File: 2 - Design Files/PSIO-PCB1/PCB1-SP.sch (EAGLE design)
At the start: 40 parts

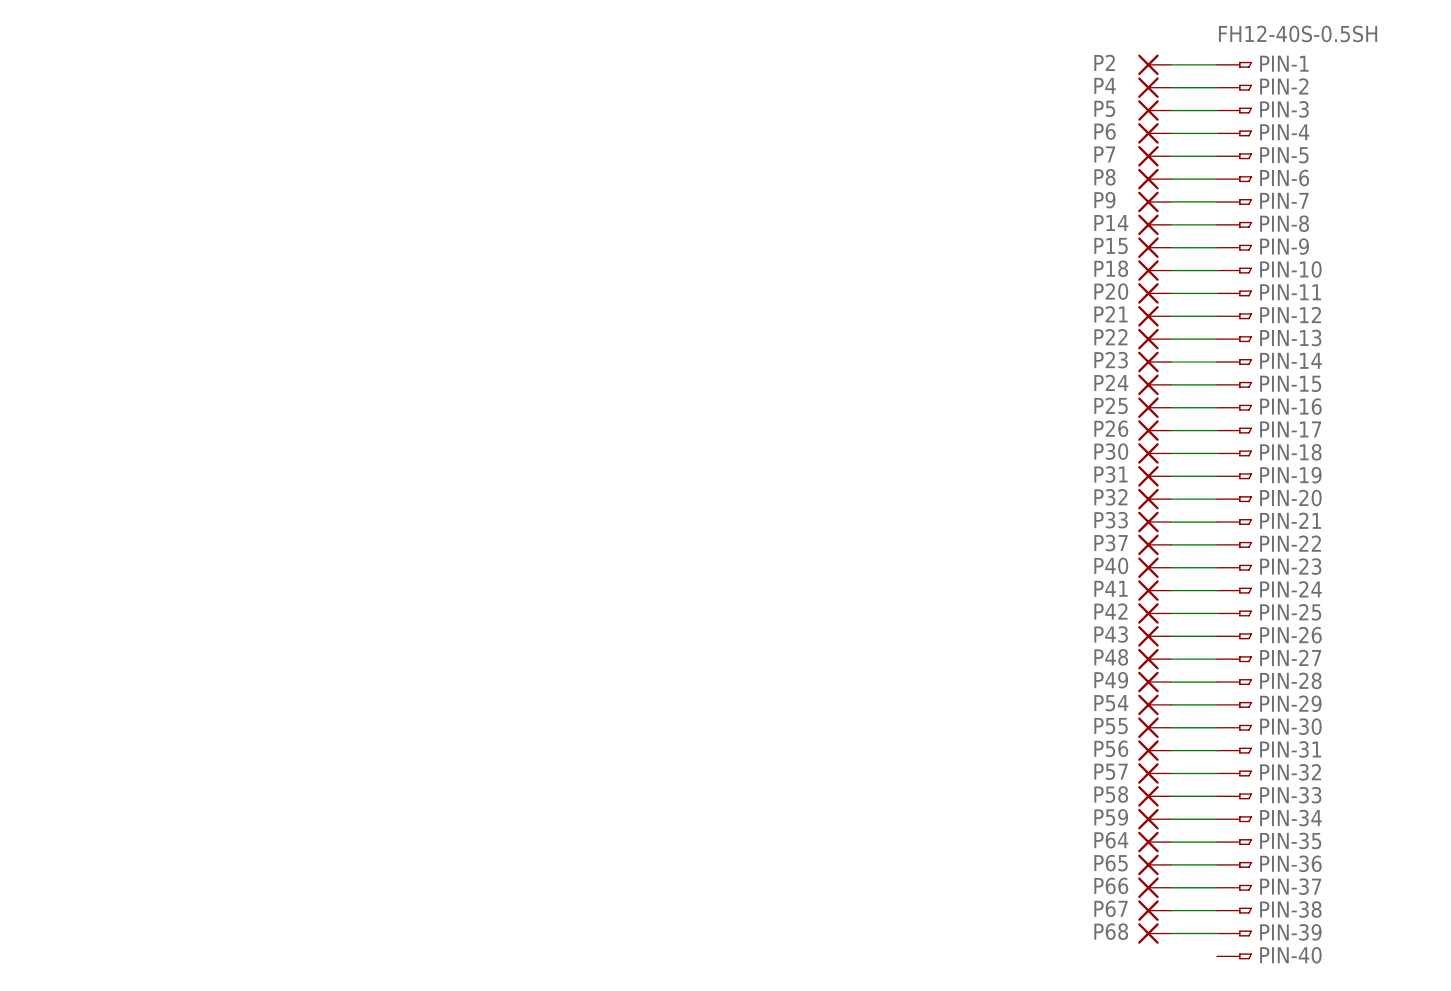
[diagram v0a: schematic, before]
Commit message: finished first PCB
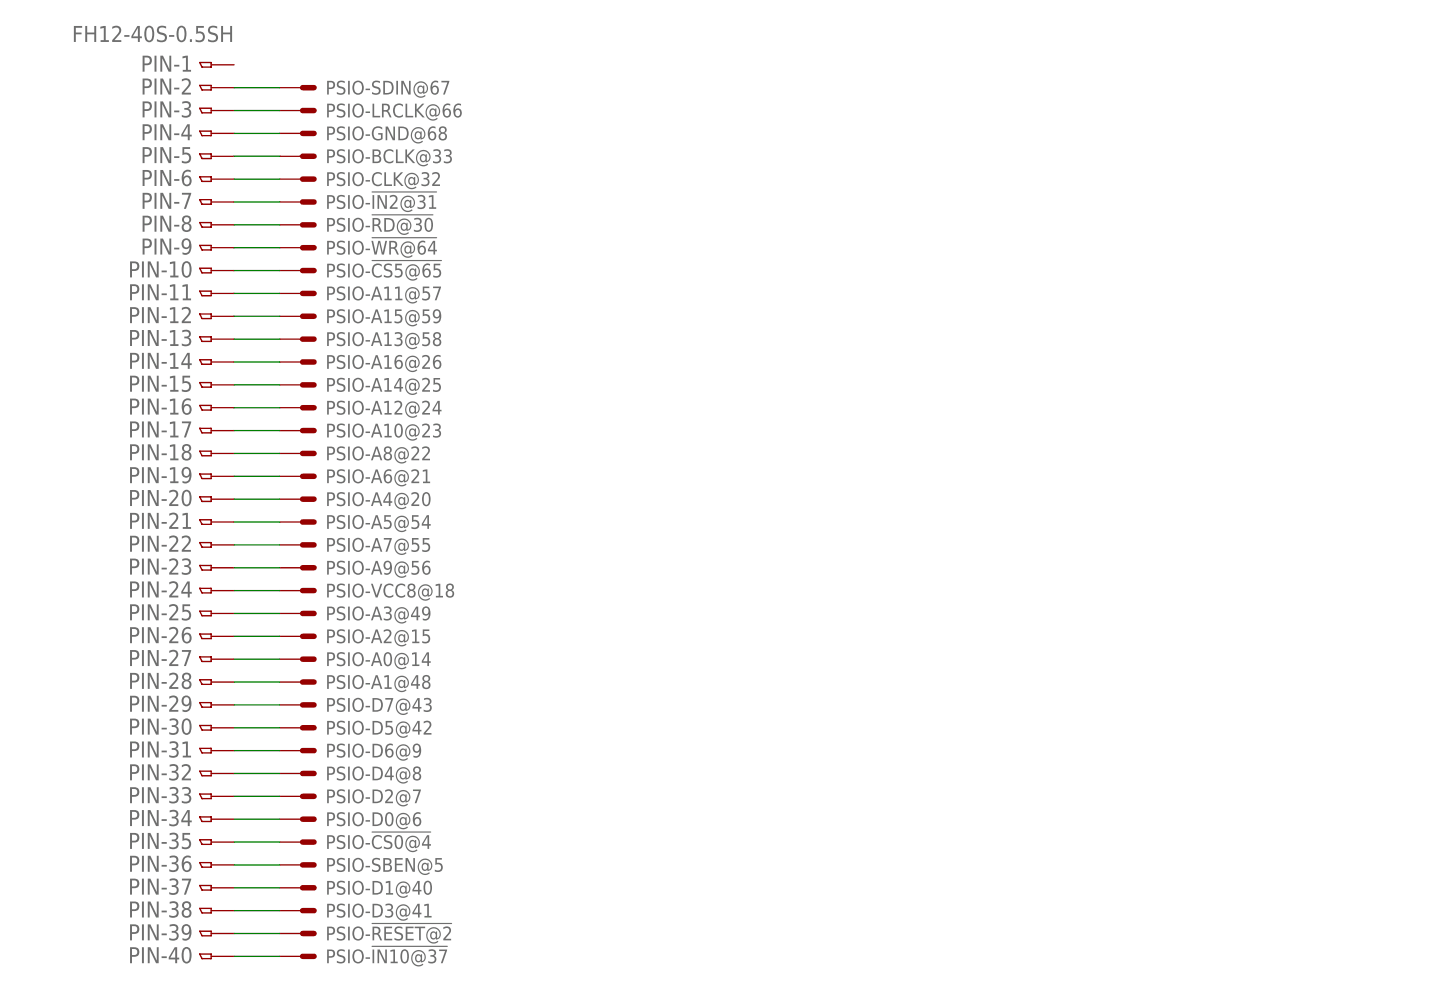
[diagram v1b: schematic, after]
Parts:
- removed P14, P15, P18, P2, P20, P21, P22, P23, P24, P25, P26, P30, P31, P32, P33, P37, P4, P40, P41, P42, P43, P48, P49, P5, P54, P55, P56, P57, P58, P59, P6, P64, P65, P66, P67, P68, P7, P8, P9: (no value), wirepad:1,6/0,8
- added PSIO: PIOCONNPIOCONN-S, pixel:PIOCONNPIOCONN-S
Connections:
- net N$1: now also PIN-40.1, PSIO-!IN10@37.S; no longer P2.P, PIN-1.1
- net N$10: now also PIN-31.1, PSIO-D6@9.S; no longer P14.P, PIN-8.1
- net N$11: now also PIN-30.1, PSIO-D5@42.S; no longer P15.P, PIN-9.1
- net N$12: now also PIN-29.1, PSIO-D7@43.S; no longer P18.P, PIN-10.1
- net N$13: now also PIN-28.1, PSIO-A1@48.S; no longer P20.P, PIN-11.1
- net N$14: now also PIN-27.1, PSIO-A0@14.S; no longer P21.P, PIN-12.1
- net N$15: now also PIN-26.1, PSIO-A2@15.S; no longer P23.P, PIN-14.1
- net N$16: now also PIN-25.1, PSIO-A3@49.S; no longer P24.P, PIN-15.1
- net N$17: now also PIN-24.1, PSIO-VCC8@18.S; no longer P25.P, PIN-16.1
- net N$18: now also PIN-2.1, PSIO-SDIN@67.S; no longer P26.P, PIN-17.1
- net N$19: now also PIN-3.1, PSIO-LRCLK@66.S; no longer P30.P, PIN-18.1
- net N$2: now also PIN-39.1, PSIO-!RESET@2.S; no longer P6.P, PIN-4.1
- net N$20: now also PIN-4.1, PSIO-GND@68.S; no longer P31.P, PIN-19.1
- net N$21: now also PIN-5.1, PSIO-BCLK@33.S; no longer P32.P, PIN-20.1
- net N$22: now also PIN-6.1, PSIO-CLK@32.S; no longer P33.P, PIN-21.1
- net N$23: now also PIN-7.1, PSIO-!IN2@31.S; no longer P37.P, PIN-22.1
- net N$24: now also PIN-8.1, PSIO-!RD@30.S; no longer P40.P, PIN-23.1
- net N$25: now also PIN-9.1, PSIO-!WR@64.S; no longer P41.P, PIN-24.1
- net N$26: now also PIN-10.1, PSIO-!CS5@65.S; no longer P48.P, PIN-27.1
- net N$27: now also PIN-23.1, PSIO-A9@56.S; no longer P49.P, PIN-28.1
- net N$28: now also PIN-11.1, PSIO-A11@57.S; no longer P54.P, PIN-29.1
- net N$29: now also PIN-22.1, PSIO-A7@55.S; no longer P55.P, PIN-30.1
- net N$3: now also PIN-38.1, PSIO-D3@41.S; no longer P42.P, PIN-25.1
- net N$30: now also PIN-21.1, PSIO-A5@54.S; no longer P56.P, PIN-31.1
- net N$31: now also PIN-12.1, PSIO-A15@59.S; no longer P57.P, PIN-32.1
- net N$32: now also PIN-13.1, PSIO-A13@58.S; no longer P58.P, PIN-33.1
- net N$33: now also PIN-20.1, PSIO-A4@20.S; no longer P59.P, PIN-34.1
- net N$34: now also PIN-14.1, PSIO-A16@26.S; no longer P64.P, PIN-35.1
- net N$35: now also PIN-19.1, PSIO-A6@21.S; no longer P65.P, PIN-36.1
- net N$36: now also PIN-15.1, PSIO-A14@25.S; no longer P66.P, PIN-37.1
- net N$37: now also PIN-16.1, PSIO-A12@24.S; no longer P67.P, PIN-38.1
- net N$38: now also PIN-17.1, PSIO-A10@23.S; no longer P68.P, PIN-39.1
- net N$39: now also PIN-18.1, PSIO-A8@22.S; no longer P43.P, PIN-26.1
- net N$4: now also PIN-37.1, PSIO-D1@40.S; no longer P22.P, PIN-13.1
- net N$5: now also PIN-36.1, PSIO-SBEN@5.S; no longer P4.P, PIN-2.1
- net N$6: now also PIN-35.1, PSIO-!CS0@4.S; no longer P5.P, PIN-3.1
- net N$7: now also PIN-34.1, PSIO-D0@6.S; no longer P7.P, PIN-5.1
- net N$8: now also PIN-33.1, PSIO-D2@7.S; no longer P8.P, PIN-6.1
- net N$9: now also PIN-32.1, PSIO-D4@8.S; no longer P9.P, PIN-7.1
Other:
- moved on the sheet: PIN-1, PIN-10, PIN-11, PIN-12, PIN-13, PIN-14, PIN-15, PIN-16, PIN-17, PIN-18, PIN-19, PIN-2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
